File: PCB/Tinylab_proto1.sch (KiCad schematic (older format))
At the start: 73 parts, among them IC1 ATXMEGA32A4U-AU, P1 SCOPE_OUT, P10 EXPANSION, P11 SWITCH, P2 USB_OTG, P3 DIG_OUT, P4 PDI/3V3, P5 SCOPE_OUT, P6 DAC_OUT, P7 PSU, P8 DIG_IN, Q1 Q_NMOS_GSD, U1 78L05, U2 LM324, U3 DMN63D8LDW, U4 DMN63D8LDW

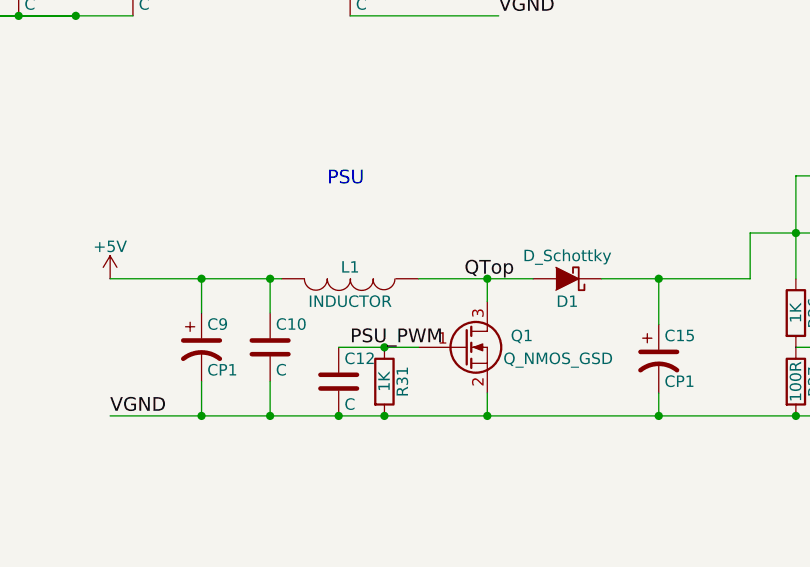
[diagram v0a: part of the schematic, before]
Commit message: New Gerbers published
Very few changes.  Fuse added, port moved.
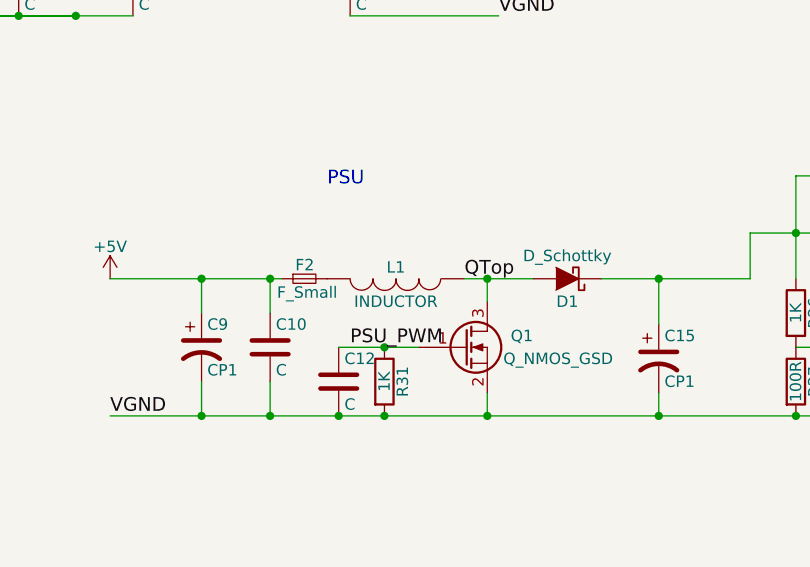
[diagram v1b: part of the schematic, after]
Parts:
- added F2: F_Small, Capacitors_SMD:C_1210, symbol F_Small
- L1: footprint Special_inductor:SELF-WE-PD-XXL -> Special_inductor:SMALL_INDUCTOR
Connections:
- net +5V: now also F2.1; no longer L1.2
- new net: F2.2, L1.2
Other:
- moved on the sheet: L1
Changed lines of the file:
@@
 L INDUCTOR L1
 U 1 1 5606EE9E
-P 10150 5050
-F 0 "L1" V 10100 5050 50  0000 C CNN
-F 1 "INDUCTOR" V 10250 5050 50  0000 C CNN
-F 2 "Special_inductor:SELF-WE-PD-XXL" H 10150 5050 60  0001 C CNN
-F 3 "" H 10150 5050 60  0000 C CNN
-	1    10150 5050
+P 10350 5050
+F 0 "L1" V 10300 5050 50  0000 C CNN
+F 1 "INDUCTOR" V 10450 5050 50  0000 C CNN
+F 2 "Special_inductor:SMALL_INDUCTOR" H 10350 5050 60  0001 C CNN
+F 3 "" H 10350 5050 60  0000 C CNN
+	1    10350 5050
 	0    1    1    0
 $EndComp
@@
 Connection ~ 10750 5050
 Wire Wire Line
-	10450 5050 10950 5050
-Wire Wire Line
 	9850 5050 9100 5050
 Wire Wire Line
@@
 	8200 3600 9200 3600
 Connection ~ 10100 5650
+Wire Wire Line
+	10950 5050 10650 5050
+$Comp
+L F_Small F2
+U 1 1 58F5AF9C
+P 9950 5050
+F 0 "F2" H 9910 5110 50  0000 L CNN
+F 1 "F_Small" H 9830 4990 50  0000 L CNN
+F 2 "Capacitors_SMD:C_1210" H 9950 5050 50  0001 C CNN
+F 3 "" H 9950 5050 50  0000 C CNN
+	1    9950 5050
+	1    0    0    -1
+$EndComp
 $EndSCHEMATC
